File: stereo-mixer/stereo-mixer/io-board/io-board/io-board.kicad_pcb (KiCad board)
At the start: 2 copper layers, 177.8 x 83.8 mm, 31 parts, among them J1 ST OUT, J10 BUS A BOARD, J11 CH B IN: L G R, J12 CH B L GAIN: TWX, J13 CH B R GAIN: TWX, J14 CH B L Level: A W B, J15 CH B R Level: A W B, J16 CH B PREAMP, J17 BUS B OUT, J18 BUS B BOARD, J19 CH C IN: L G R, J2 MIXER BOARD, J20 CH C L GAIN: TWX, J21 CH C R GAIN: TWX, J22 CH C L Level: A W B, J23 CH C R Level: A W B, J24 CH C PREAMP, J25 CH D IN: L G R, J26 CH D L GAIN: TWX, J27 CH D R GAIN: TWX, J28 CH D L Level: A W B, J29 CH D R Level: A W B, J3 CH A IN: L G R, J30 CH D PREAMP, J31 -15V GND +15V, J4 CH A L GAIN: TWX, J5 CH A R GAIN: TWX, J6 CH A L Level: A W B, J7 CH A R Level: A W B, J8 CH A PREAMP, J9 BUS A OUT

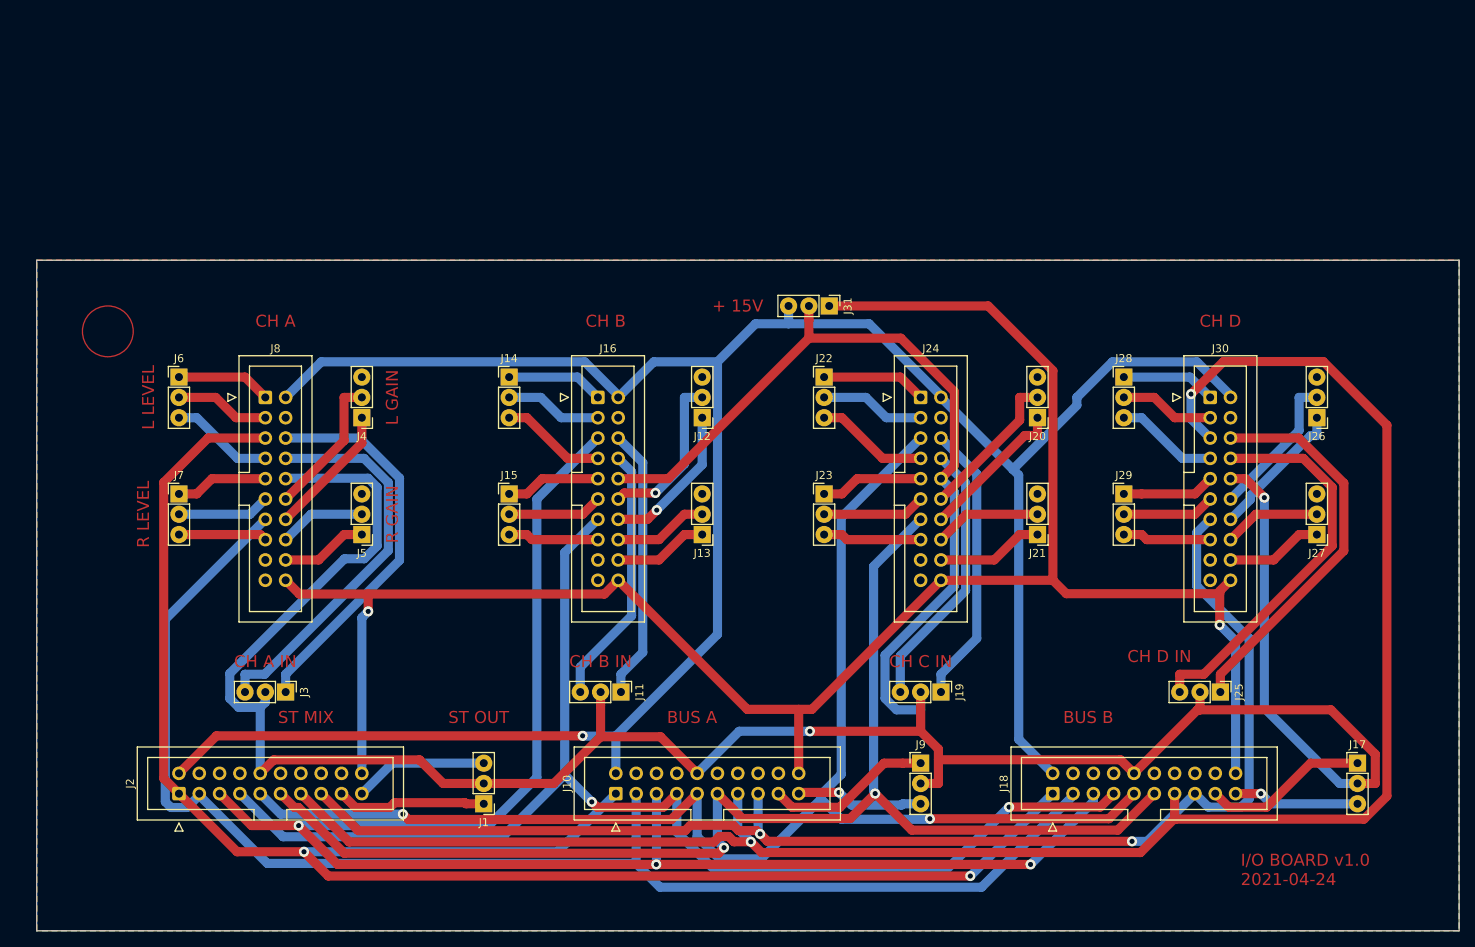
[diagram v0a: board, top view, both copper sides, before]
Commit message: updated for cnc
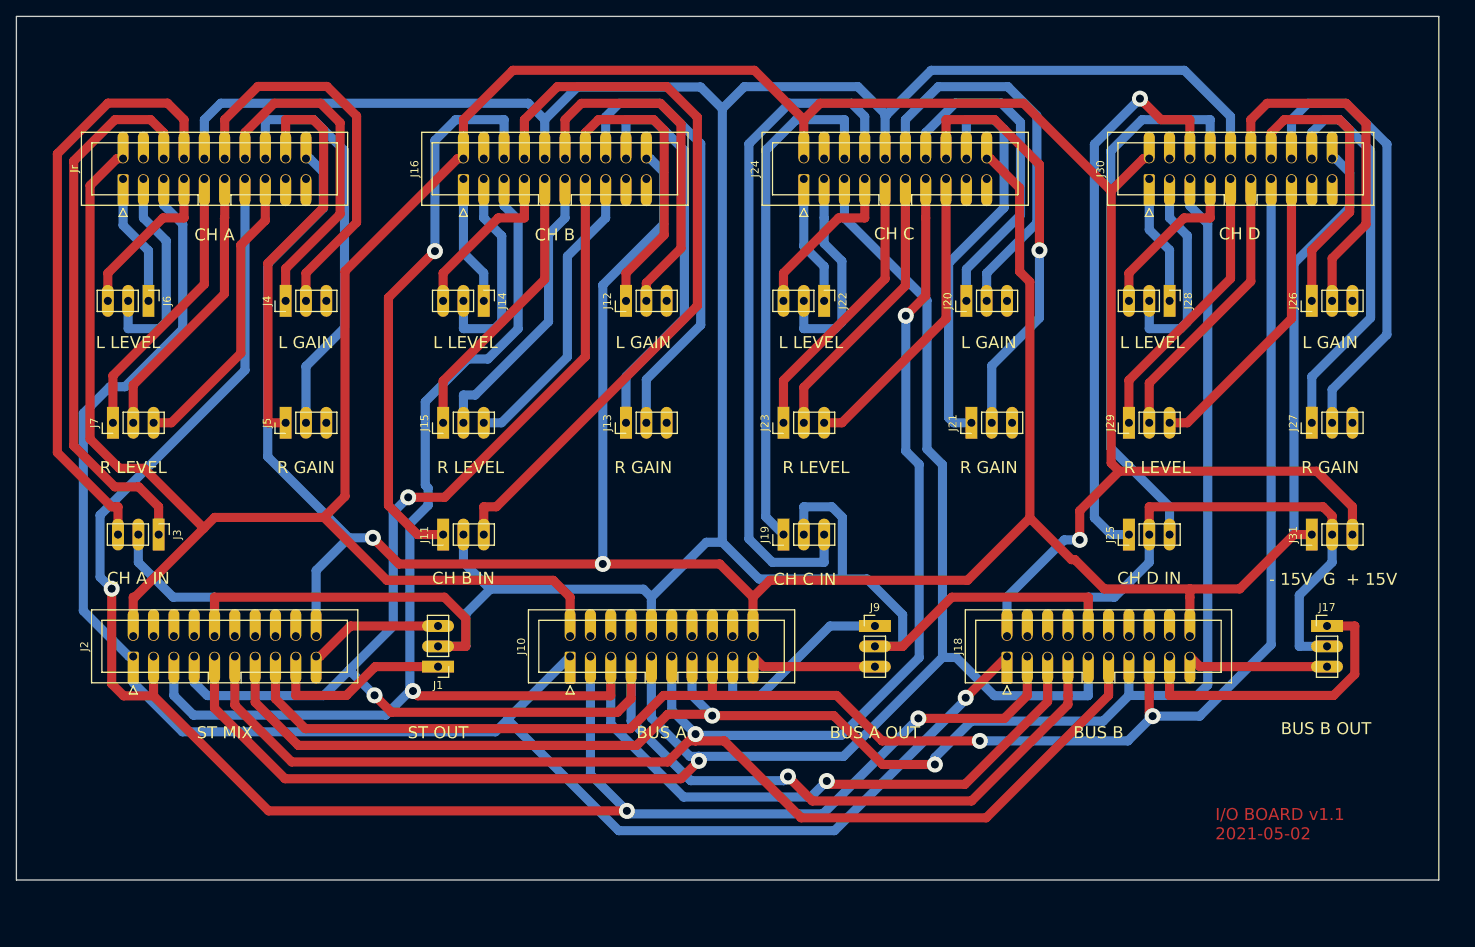
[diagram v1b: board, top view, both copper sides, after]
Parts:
- moved J31 66.8 mm to (212.7, 83.8), turned to 90 degrees
- moved Jr 32.6 mm to (64.1, 39.4), turned to 90 degrees
- moved J16 32.1 mm to (106.7, 39.4), turned to 90 degrees
- moved J24 31.0 mm to (149.2, 39.4), turned to 90 degrees
- moved J11 29.7 mm to (104.1, 83.8), turned to 90 degrees
- moved J30 28.3 mm to (192.4, 39.4), turned to 90 degrees
- moved J19 27.8 mm to (146.7, 83.8), turned to 90 degrees
- moved J3 25.3 mm to (68.6, 83.8)
- moved J25 22.8 mm to (189.9, 83.8), turned to 90 degrees
- moved J1 18.1 mm to (103.5, 100.3)
- moved J10 18.1 mm to (120.0, 99.1)
- moved J18 18.1 mm to (174.6, 99.1)
- moved J2 18.1 mm to (65.4, 99.1)
- moved J9 18.1 mm to (158.1, 95.2)
- moved J17 17.6 mm to (214.6, 95.2)
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- renumbered J8 to Jr
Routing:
- net /-_15V: track 246.0 -> 370.2 mm
- net GND: track 396.0 -> 486.5 mm, vias 2 -> 0
- net /+_15V: track 297.0 -> 386.3 mm
- net /CH_C_R_OUT: track 163.7 -> 239.9 mm
- net /CH_B_R_IN: track 32.6 -> 93.9 mm
- net /CH_B_R_OUT: track 161.4 -> 222.6 mm, vias 2 -> 3
- net /CH_A_R_OUT: track 173.6 -> 229.5 mm, vias 0 -> 3
- net /CH_C_R_IN: track 33.9 -> 86.0 mm
- net /CH_B_R_GAIN_WIPER: track 11.8 -> 57.6 mm
- net /CH_D_R_GAIN_WIPER: track 12.1 -> 57.4 mm
- net /CH_D_R_OUT: track 166.1 -> 211.1 mm
- net /CH_A_R_GAIN_WIPER: track 10.8 -> 52.4 mm
- net /CH_A_R_GAIN_TERM_A: track 10.8 -> 51.9 mm
- net /CH_C_R_GAIN_WIPER: track 13.4 -> 53.6 mm, vias 0 -> 1
- net /CH_C_L_OUT: track 174.2 -> 213.3 mm, vias 2 -> 1
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- removed copper zone on B.Cu, net (none)
- removed copper zone on F.Cu, net (none)
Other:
- board size 177.8 x 83.8 mm -> 177.8 x 108 mm
- net class Default: clearance 0.254 -> 1; trace_width 1.143 -> 1; via_dia 0.8 -> 2; via_drill 0.4 -> 1
- rule trace_clearance: 0.254 -> 1
- board text added: "- 15V G + 15V"
- board text added: "BUS A OUT"
- board text added: "BUS B OUT"
- board text added: "CH C"
- board text added: "I/O BOARD v1.1 2021-05-02"
- board text removed: "+ 15V"
- board text removed: "I/O BOARD v1.0 2021-04-24"
